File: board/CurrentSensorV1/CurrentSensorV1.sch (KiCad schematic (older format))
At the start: 17 parts, among them J1 USB_B_Micro, J2 FTDI_Header, J3 AudioJack3_GroundPinNumbers, J4 0, J5 0, J6 Conn_01x02_Female, J7 Conn_01x02_Female, SW2 SW_SPST_SM_DP, SW3 SW_SPST_SM_DP, U1 UA78M05CDCY, U2 ESP-01v090, U3 ADS1115

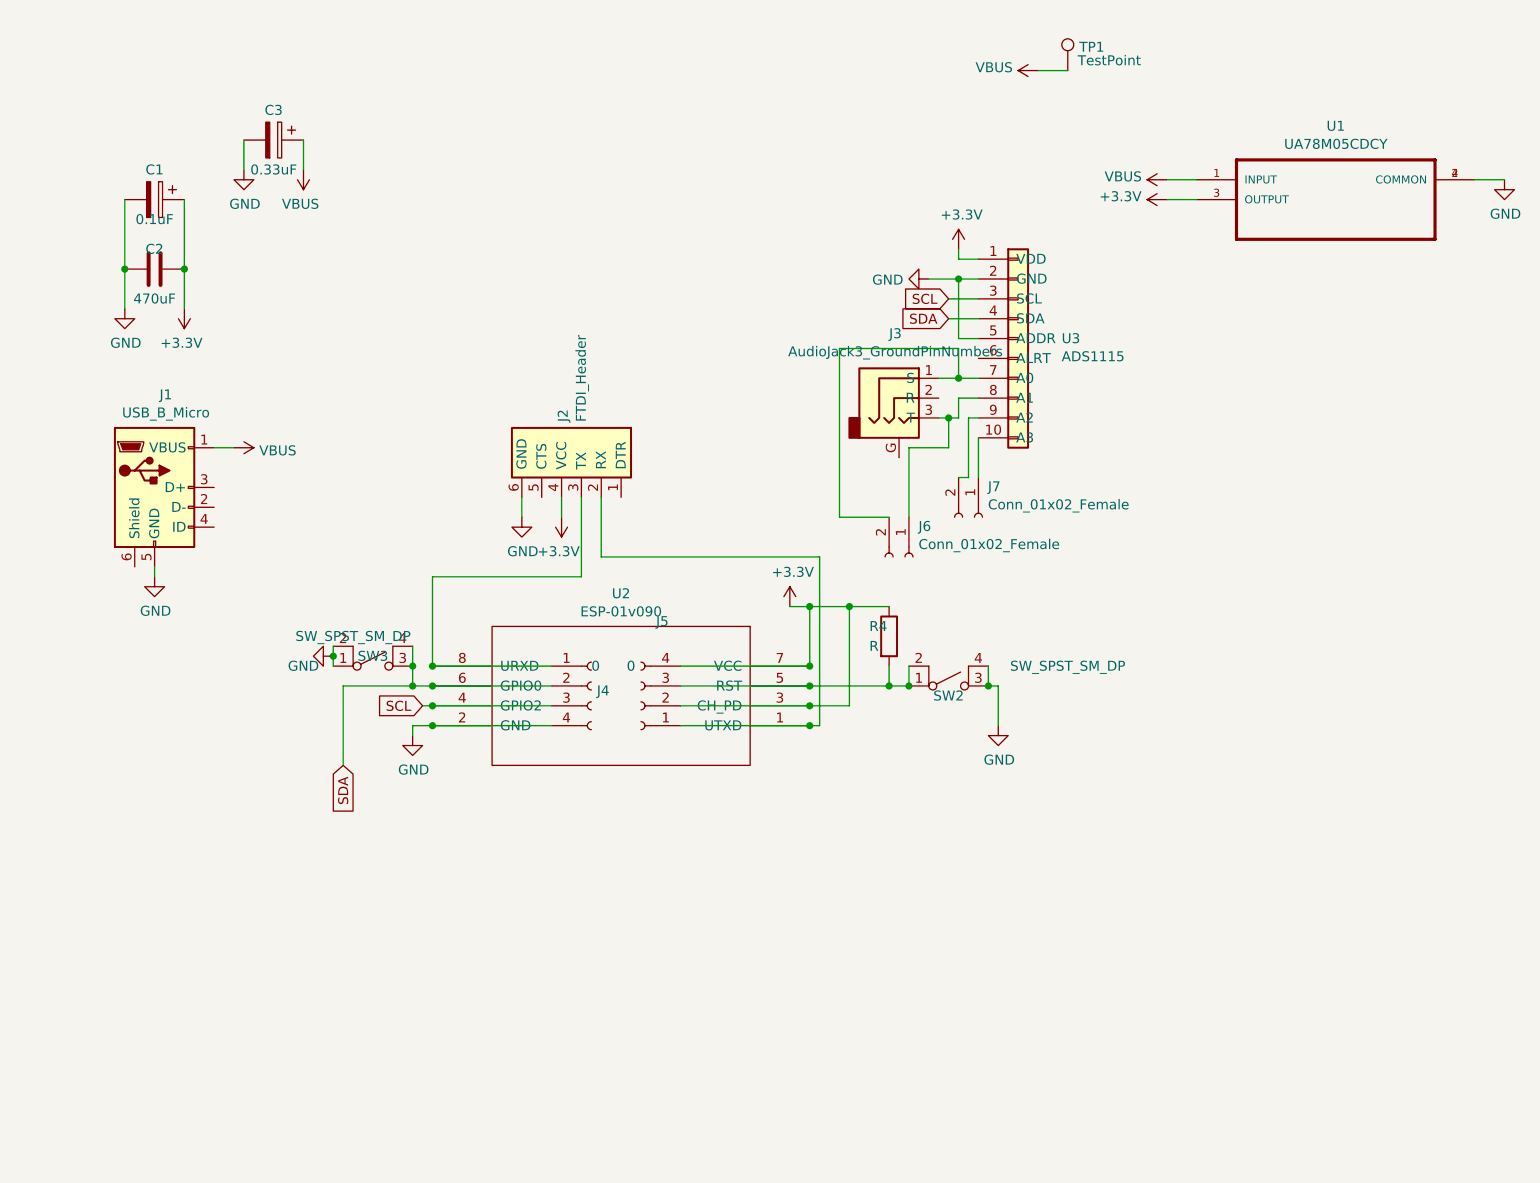
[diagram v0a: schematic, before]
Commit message: Starting v4
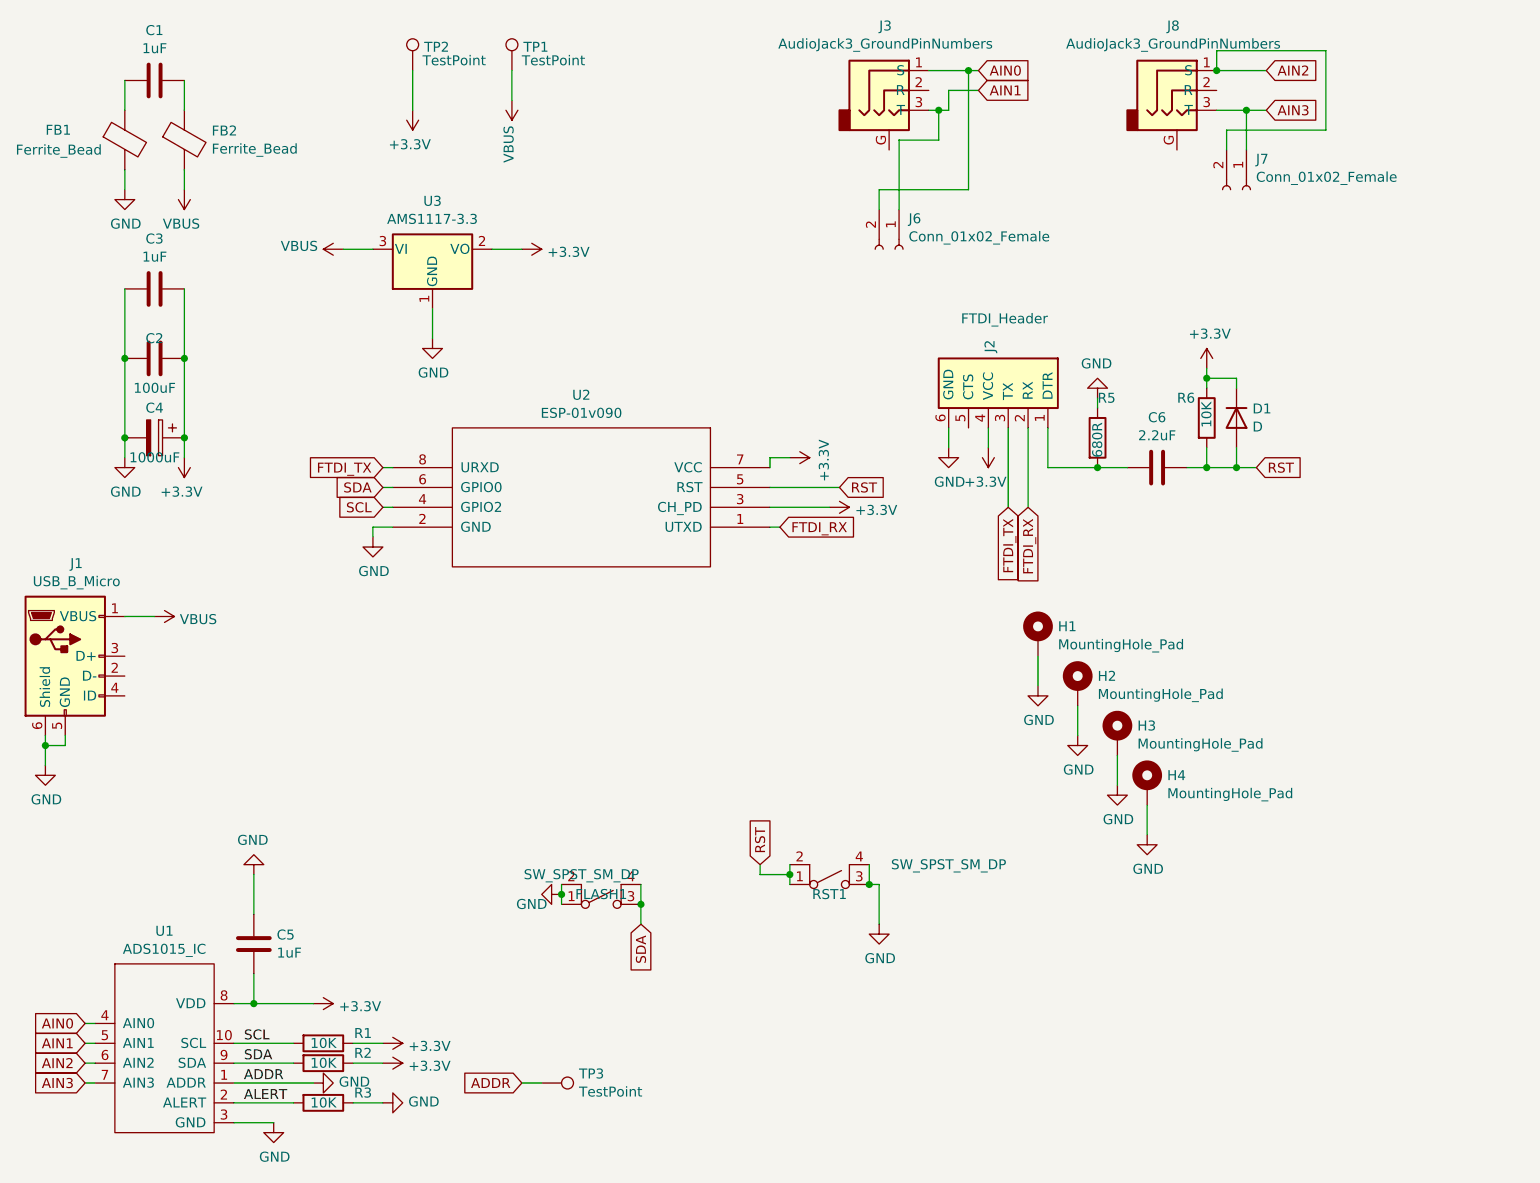
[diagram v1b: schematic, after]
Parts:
- removed C1: 0.1uF, Capacitor_THT:C_Disc_D3.0mm_W1.6mm_P2.50mm, symbol Device:CP
- removed C3: 0.33uF, Capacitor_THT:C_Disc_D3.0mm_W1.6mm_P2.50mm, symbol Device:CP
- removed J4, J5: 0, Connector_PinHeader_2.54mm:PinHeader_1x04_P2.54mm_Vertical, symbol Connector:Conn_01x04_Female
- removed R4: R, Resistor_THT:R_Axial_DIN0204_L3.6mm_D1.6mm_P7.62mm_Horizontal, symbol Device:R
- removed U1: UA78M05CDCY, UA78M05CDCY:SOT230P700X180-4N, symbol UA78M05CDCY:UA78M05CDCY
- removed U3: ADS1115, Connector_PinHeader_2.54mm:PinHeader_1x10_P2.54mm_Vertical, symbol ADS1115:ADS1115
- added C1, C3, C5: 1uF, Capacitor_SMD:C_0402_1005Metric, symbol Device:C
- added C4: 1000uF, Capacitor_SMD:C_Elec_8x10.2, symbol Device:CP
- added C6: 2.2uF, Capacitor_SMD:C_0603_1608Metric, symbol Device:C
- added D1: D, Diode_SMD:D_SOD-123, symbol Device:D
- added FB1, FB2: Ferrite_Bead, Resistor_SMD:R_0805_2012Metric, symbol Device:Ferrite_Bead
- added H1, H2, H3, H4: MountingHole_Pad, MountingHole:MountingHole_2.5mm_Pad, symbol Mechanical:MountingHole_Pad
- added J8: AudioJack3_GroundPinNumbers, audio35mm:Tayda_3.5mm_stereo_TRS_jack_A-853, symbol JACK_TRS:AudioJack3_GroundPinNumbers
- added R1, R2, R3, R6: 10K, Resistor_SMD:R_0603_1608Metric, symbol Device:R
- added R5: 680R, Resistor_SMD:R_0603_1608Metric, symbol Device:R
- added TP2, TP3: TestPoint, Connector_PinSocket_2.54mm:PinSocket_1x01_P2.54mm_Vertical, symbol Connector:TestPoint
- added U1: ADS1015_IC, Package_SO:VSSOP-10_3x3mm_P0.5mm, symbol ADS1115:ADS1015_IC
- added U3: AMS1117-3.3, Package_TO_SOT_SMD:SOT-223-3_TabPin2, symbol Regulator_Linear:AMS1117-3.3
- C2: value 470uF -> 100uF; footprint Capacitor_THT:CP_Radial_D5.0mm_P2.00mm -> Capacitor_Tantalum_SMD:CP_EIA-3528-12_Kemet-T; JLCPCB_CORRECTION (none) -> 0;0;180; LCSC (none) -> C16133
- FLASH1: renamed from SW3; LCSC (none) -> C530667
- RST1: renamed from SW2; LCSC (none) -> C530667
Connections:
- net +3V3: now also C3.1, C4.1, C5.2, D1.1 (K), R1.1, R2.1, R6.1, TP2.1, U1.8 (VDD), U3.2 (VO)
- net GND: now also J1.6 (Shield), C3.2, C4.2, C5.1, FB1.2, H1.1, H2.1, H3.1, H4.1, R3.1, R5.1, TP3.1, U1.1 (ADDR), U1.3 (GND), U3.1 (GND)
- net SCL: now also R1.2, U1.10 (SCL)
- net SDA: now also R2.2, U1.9 (SDA)
- net VBUS: now also FB2.2, U3.3 (VI)
- net FTDI_RX: now reaches J2.2 (RX), U2.1 (UTXD)
- net RST: now reaches RST1.1 (A), RST1.2 (A), U2.5 (RST)
- net RST: now also C6.1, D1.2 (A), R6.2
- net FTDI_TX: now reaches J2.3 (TX), U2.8 (URXD)
- net at J2.1 (DTR): now also C6.2, R5.2
- net AIN3: now reaches J7.1 (Pin_1)
- net AIN3: now also J8.3 (T), U1.7 (AIN3)
- net AIN2: now reaches J7.2 (Pin_2)
- net AIN2: now also J8.1 (S), U1.6 (AIN2)
- net AIN0: now reaches J3.1 (S), J6.2 (Pin_2)
- net AIN0: now also U1.4 (AIN0)
- net AIN1: now reaches J3.3 (T), J6.1 (Pin_1)
- net AIN1: now also U1.5 (AIN1)
- new net: C1.1, FB2.1
- new net: C1.2, FB1.1
- new net ALERT: R3.2, U1.2 (ALERT)
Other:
- moved on the sheet: C2, FLASH1, J2, J3, J6, J7, RST1, TP1, U2
